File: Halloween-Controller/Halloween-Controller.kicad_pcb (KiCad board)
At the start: 2 copper layers, 63.5 x 43.2 mm, 30 parts, among them IC1 ATmega328_B, J1 Neopixel_A, J2 Conn_FTDI, J3 Conn_Sensors, J4 Neopixel_B, J5 Neopixel_C, J6 Conn_Exp, J7 Neopixel_D, J8 Conn_GPIO_IN, SW1 SW_SPST, Y1 16MHz

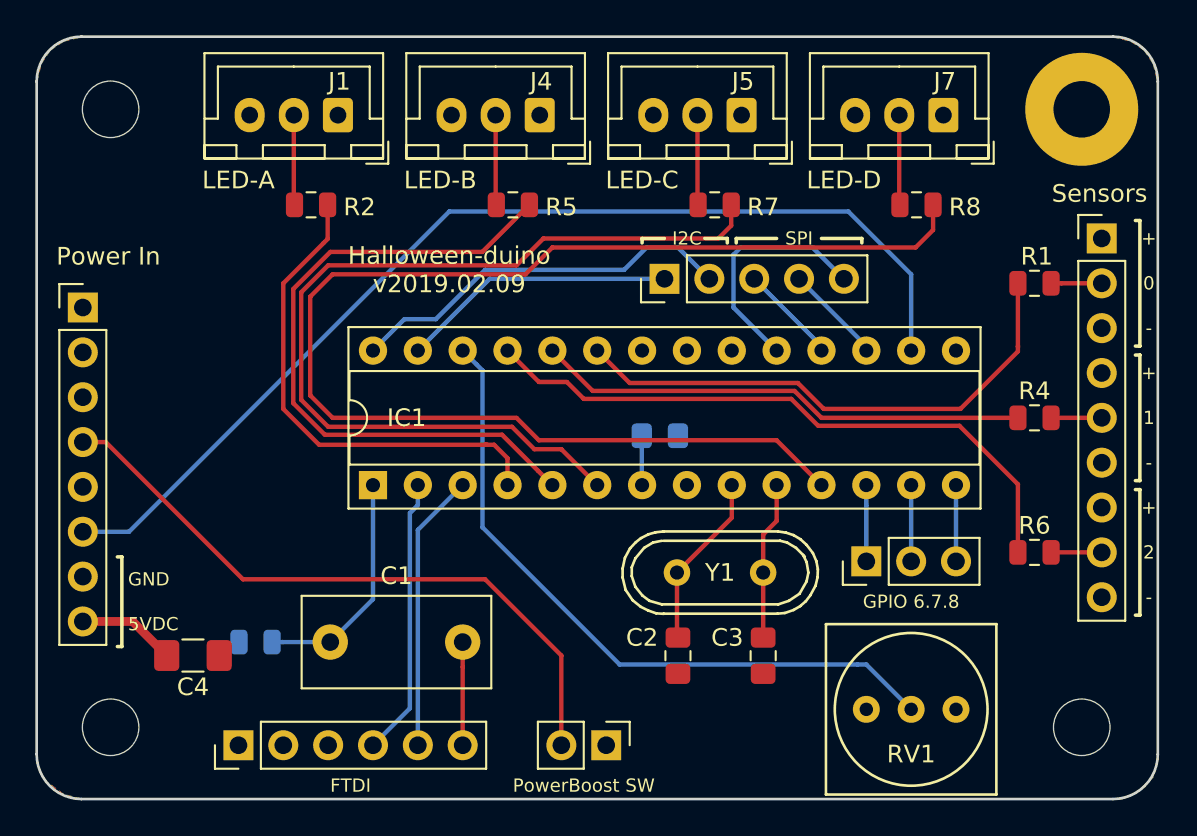
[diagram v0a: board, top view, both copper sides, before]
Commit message: WIP....
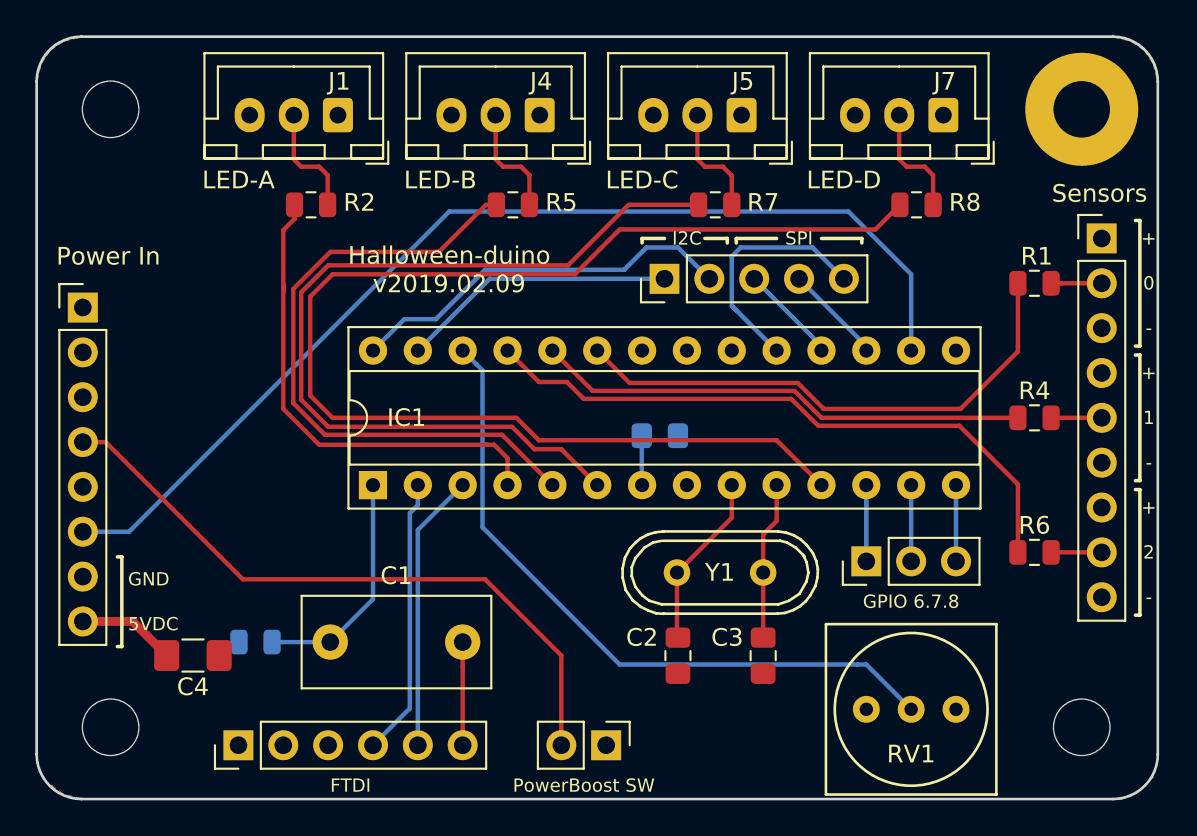
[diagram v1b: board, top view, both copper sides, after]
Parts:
- turned R7 to 180 degrees
- turned R2 to 180 degrees
- turned R5 to 180 degrees
- turned R8 to 180 degrees
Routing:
- net /GPIO_5: track 74.9 -> 72.2 mm
- net /GPIO_4: track 52.0 -> 49.5 mm
- net /GPIO_3: track 38.4 -> 36.6 mm
- net Net-(J5-Pad2): track 5.10 -> 6.48 mm
- net Net-(J1-Pad2): track 5.10 -> 6.47 mm
- net Net-(J7-Pad2): track 5.10 -> 6.47 mm
- net Net-(J4-Pad2): track 5.10 -> 6.47 mm
